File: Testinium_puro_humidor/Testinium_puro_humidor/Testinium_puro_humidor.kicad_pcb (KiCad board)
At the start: 2 copper layers, 44.5 x 70.2 mm, 34 parts, among them J1 Conn_01x02_Fan1, J2 Conn_01x02_Fan1, J3 Piezzo, J4 Power_Conn, J5 Conn_01x02_Fan1, J6 Conn_01x04_Pin, Q1 2N3904, Q3 IRLML6344TRPBF, Q5 IRLML6344TRPBF, U1 LD1117S33TR_SOT223, U2 ESP32-DEVKITC-32D, U3 TPS54202DDC, U4 PC817

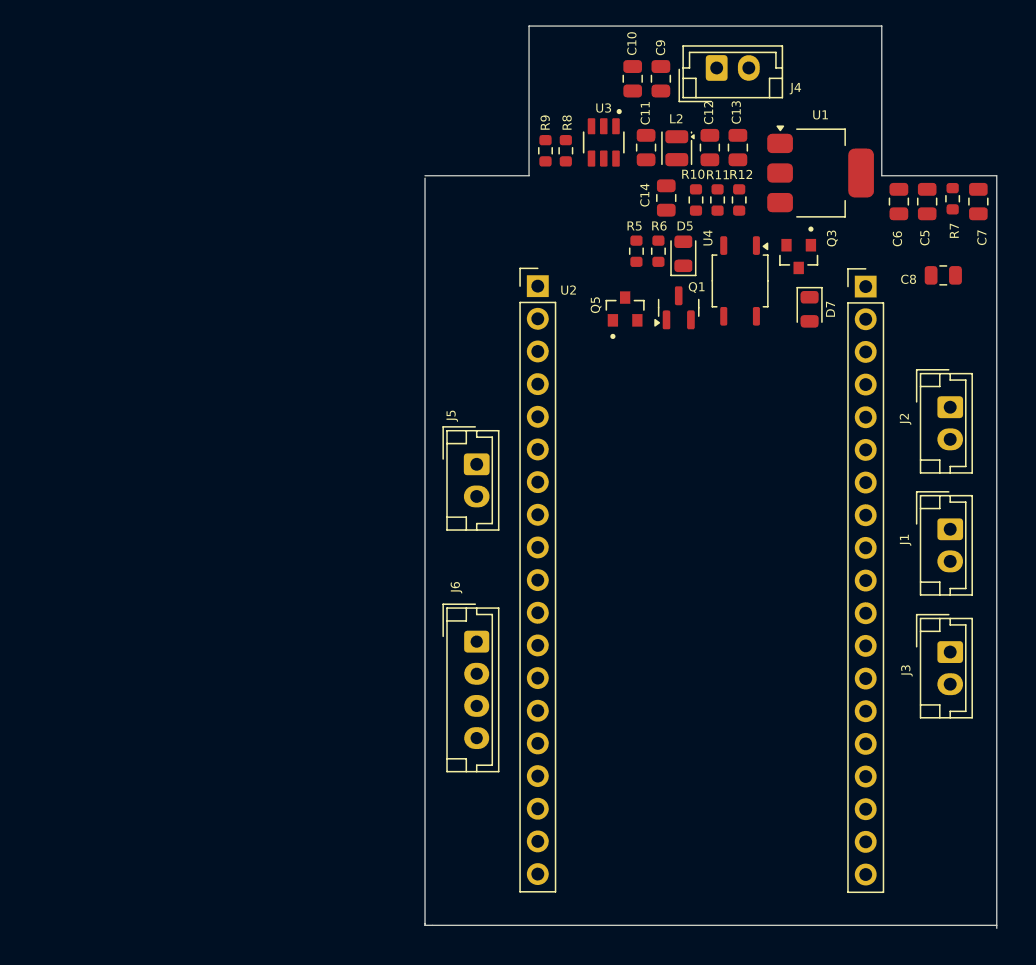
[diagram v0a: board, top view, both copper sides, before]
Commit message: sematik tamamlandi
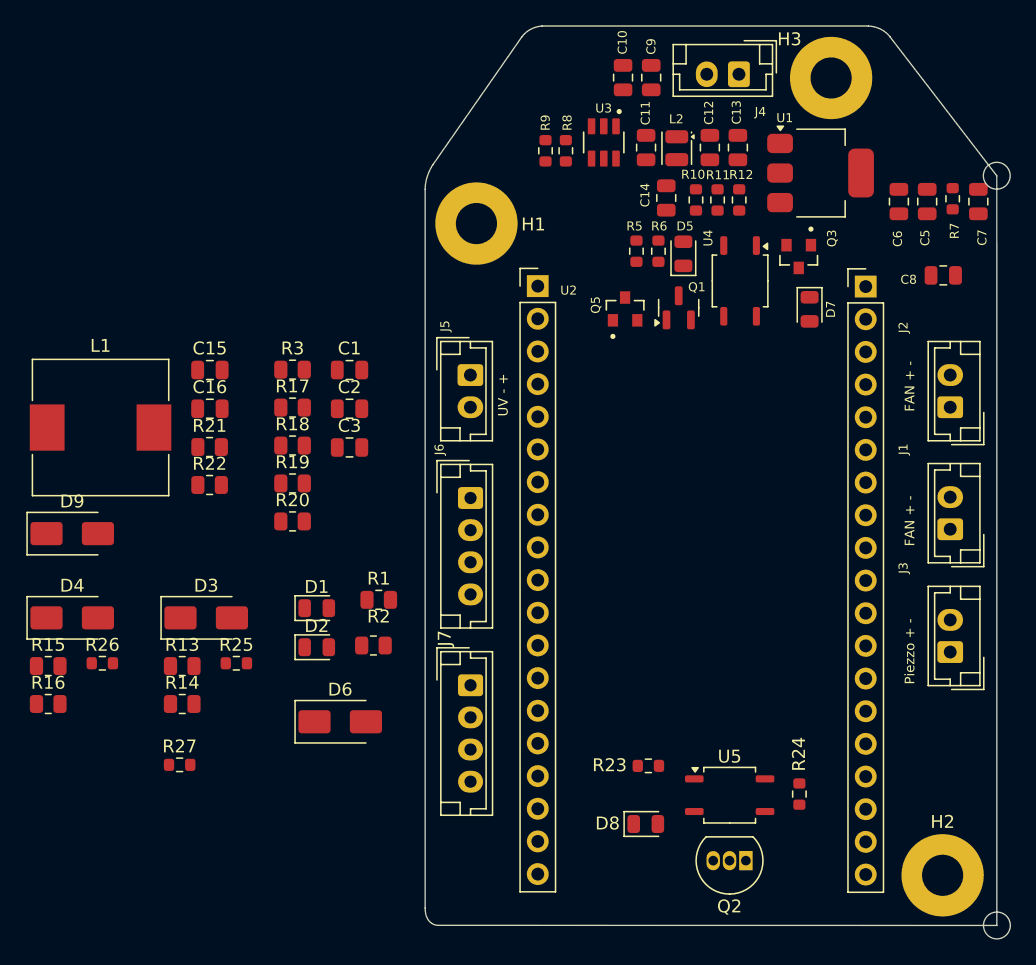
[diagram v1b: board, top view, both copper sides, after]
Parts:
- added C1: 22uF / 25v, Capacitor_SMD:C_0805_2012Metric, F.Cu at (57.5, 42.9)
- added C15: 47nF, Capacitor_SMD:C_0805_2012Metric, F.Cu at (46.6, 42.9)
- added C16: 47nF, Capacitor_SMD:C_0805_2012Metric, F.Cu at (46.6, 45.9)
- added C2: 0.1uF / 25v, Capacitor_SMD:C_0805_2012Metric, F.Cu at (57.5, 45.9)
- added C3: 0.1uF / 25v, Capacitor_SMD:C_0805_2012Metric, F.Cu at (57.5, 48.9)
- added D1: GreenLed, LED_SMD:LED_0805_2012Metric, F.Cu at (54.9, 61.4)
- added D2: RedLed, LED_SMD:LED_0805_2012Metric, F.Cu at (54.9, 64.4)
- added D3: D, Diode_SMD:D_SMA, F.Cu at (46.3, 62.1)
- added D4: D, Diode_SMD:D_SMA, F.Cu at (35.9, 62.1)
- added D6: D, Diode_SMD:D_SMA, F.Cu at (56.8, 70.2)
- added D8: GreenLed, LED_SMD:LED_0805_2012Metric, F.Cu at (80.5, 78.2)
- added D9: D, Diode_SMD:D_SMA, F.Cu at (35.9, 55.6)
- added H1: MountingHole_Pad_MP, MountingHole:MountingHole_3.2mm_M3_Pad, F.Cu at (67.3, 31.5)
- added H2: MountingHole_Pad_MP, MountingHole:MountingHole_3.2mm_M3_Pad, F.Cu at (103.6, 82.2)
- added H3: MountingHole_Pad_MP, MountingHole:MountingHole_3.2mm_M3_Pad, F.Cu at (94.9, 20.1)
- added J7: Conn_Oled, Connector_JST:JST_EH_B4B-EH-A_1x04_P2.50mm_Vertical, F.Cu at (66.9, 67.4)
- added L1: 100mH, Inductor_SMD:L_10.4x10.4_H4.8, F.Cu at (38.1, 47.3)
- added Q2: 2SC5200, Package_TO_SOT_THT:TO-92_Inline, F.Cu at (88.3, 81.0)
- added R1: 330R, Resistor_SMD:R_0805_2012Metric, F.Cu at (59.8, 60.7)
- added R13: 150R, Resistor_SMD:R_0805_2012Metric, F.Cu at (44.5, 65.9)
- added R14: 10K, Resistor_SMD:R_0805_2012Metric, F.Cu at (44.5, 68.8)
- added R15: 10K, Resistor_SMD:R_0805_2012Metric, F.Cu at (34.0, 65.9)
- added R16: 150R, Resistor_SMD:R_0805_2012Metric, F.Cu at (34.0, 68.8)
- added R17: 4K7, Resistor_SMD:R_0805_2012Metric, F.Cu at (53.0, 45.8)
- added R18: 4K7, Resistor_SMD:R_0805_2012Metric, F.Cu at (53.0, 48.7)
- added R19: 4K7, Resistor_SMD:R_0805_2012Metric, F.Cu at (53.0, 51.7)
- added R2: 330R, Resistor_SMD:R_0805_2012Metric, F.Cu at (59.3, 64.3)
- added R20: 4K7, Resistor_SMD:R_0805_2012Metric, F.Cu at (53.0, 54.6)
- added R21: 2K2, Resistor_SMD:R_0805_2012Metric, F.Cu at (46.6, 48.9)
- added R22: 4R7, Resistor_SMD:R_0805_2012Metric, F.Cu at (46.6, 51.8)
- added R23: 330R, Resistor_SMD:R_0603_1608Metric, F.Cu at (80.7, 73.6)
- added R24: 100R, Resistor_SMD:R_0603_1608Metric, F.Cu at (92.5, 75.8)
- added R25: 0R, Resistor_SMD:R_0603_1608Metric, F.Cu at (48.7, 65.7)
- added R26: 0R, Resistor_SMD:R_0603_1608Metric, F.Cu at (38.3, 65.7)
- added R27: 0R, Resistor_SMD:R_0603_1608Metric, F.Cu at (44.3, 73.6)
- added R3: 10k, Resistor_SMD:R_0805_2012Metric, F.Cu at (53.0, 42.8)
- added U5: PC817, Package_SO:SOP-4_3.8x4.1mm_P2.54mm, F.Cu at (87.0, 75.9)
- J5: value Conn_01x02_Fan1 -> Conn_01x02_UV_LED
- J6: value Conn_01x04_Pin -> Conn_Sht31
- moved J6 11.2 mm to (66.9, 52.8)
- moved J5 6.96 mm to (66.9, 43.2)
- moved J4 1.80 mm to (87.8, 19.9), turned to 180 degrees
- moved C10 0.76 mm to (78.8, 20.1)
- moved C9 0.76 mm to (80.9, 20.1)
- turned J1 to 90 degrees
- turned J2 to 90 degrees
- turned J3 to 90 degrees
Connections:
- C10 pad 1: /regulator/12V -> Power
- C10 pad 2: GND -> Piezzo_-
- C12 pad 1: GND -> Piezzo_-
- C13 pad 1: GND -> Piezzo_-
- C5 pad 2: GND -> Piezzo_-
- C6 pad 2: GND -> Piezzo_-
- C7 pad 1: /regulator/3V3_esp32 -> VDD3
- C7 pad 2: GND -> Piezzo_-
- C8 pad 1: /regulator/3V3_esp32 -> VDD3
- C8 pad 2: GND -> Piezzo_-
- C9 pad 1: /regulator/12V -> Power
- C9 pad 2: GND -> Piezzo_-
- D7 pad 1: GND -> Piezzo_-
- D7 pad 2: /regulator/3V3_esp32 -> VDD3
- J3 pad 1: unconnected-(J3-Pin_1-Pad1) -> piezzo_pin1
- J3 pad 2: GND -> Piezzo_-
- J4 pad 1: /regulator/12V -> Piezzo_-
- J4 pad 2: GND -> Power
- J5 pad 1: /uvled/3V3 -> UV_LED_+
- J5 pad 2: GND -> UV_LED_+
- J6 pad 1: /sht31/Sht31_3V3 -> Net-(J6-Pin_1)
- J6 pad 2: /sht31/Sht31_SDA -> /ESP32/I2C1_SDA
- J6 pad 3: /sht31/Sht31_SCL -> /ESP32/I2C1_SCL
- J6 pad 4: /sht31/Sht31_GND -> Piezzo_-
- Q1 pad 1: GND -> Piezzo_-
- Q3 pad 2: GND -> Piezzo_-
- Q5 pad 2: GND -> Piezzo_-
- R12 pad 1: GND -> Piezzo_-
- R5 pad 1: /uvled/3V3 -> 3V3
- R7 pad 2: /regulator/3V3_esp32 -> VDD3
- R8 pad 2: /regulator/12V -> Power
- R9 pad 1: GND -> Piezzo_-
- U1 pad 1: GND -> Piezzo_-
- U2 pad J3-13: unconnected-(U2-IO4-PadJ3-13) -> /ESP32/I2C0_SCL
- U2 pad J3-14: unconnected-(U2-IO0-PadJ3-14) -> /ESP32/I2C0_SDA
- U2 pad J3-17: unconnected-(U2-SD1-PadJ3-17) -> /ESP32/I2C1_SDA
- U2 pad J3-18: unconnected-(U2-SD0-PadJ3-18) -> /ESP32/I2C1_SCL
- U3 pad 1: GND -> Piezzo_-
- U3 pad 3: /regulator/12V -> Power
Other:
- board size 44.5 x 70.2 mm -> 45.5 x 71 mm
- board text added: "FAN + -"
- board text added: "Piezzo + -"
- board text added: "UV - +"
